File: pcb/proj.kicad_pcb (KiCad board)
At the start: 2 copper layers, 125 x 185 mm, 152 parts, among them J1 Conn_02x05_Odd_Even, Q1 MMBT3904, SW1 Reset, SW10 8, SW11 9, SW12 /, SW13 Deg/Rad, SW14 Clear, SW15 4, SW16 5, SW17 6, SW18 X, SW19 Constants, SW2 Y/Stats, SW20 Del, SW21 1, SW22 2, SW23 3, SW24 -, SW25 Alpha, SW26 (/), SW27 Sin(x)/Sin-1(x), SW28 Cos(x)/Cos-1(x), SW29 Tan(x)/Tan-1(x), SW3 ./,, SW30 +, SW31 2nd, SW32 Γ(x), SW33 x^y/y√x, SW34 x^2/√x, SW35 log(x)/ln(x), SW36 e^x/10^x, SW37 Graph, SW38 Programs, SW39 Left, SW4 0, SW40 Up, SW41 Right, SW42 Down, SW43 Power, SW44 FPU BOOT0, SW45 Reset, SW5 +/-, SW6 Solve/=, SW7 Sci/Norm, SW8 X/Matrix, SW9 7, U1 PIC16C74, U2 STM32F401RCTx, U3 74HC238, U4 ISL9111EH50Z-T7A, U5 SN74LVC1G32DBVR, U6 TPS61021A, U7 SiP32510DT, U8 SN74LV1T34DBV, U9 SN74LV1T34DBV, Y1 20MHz

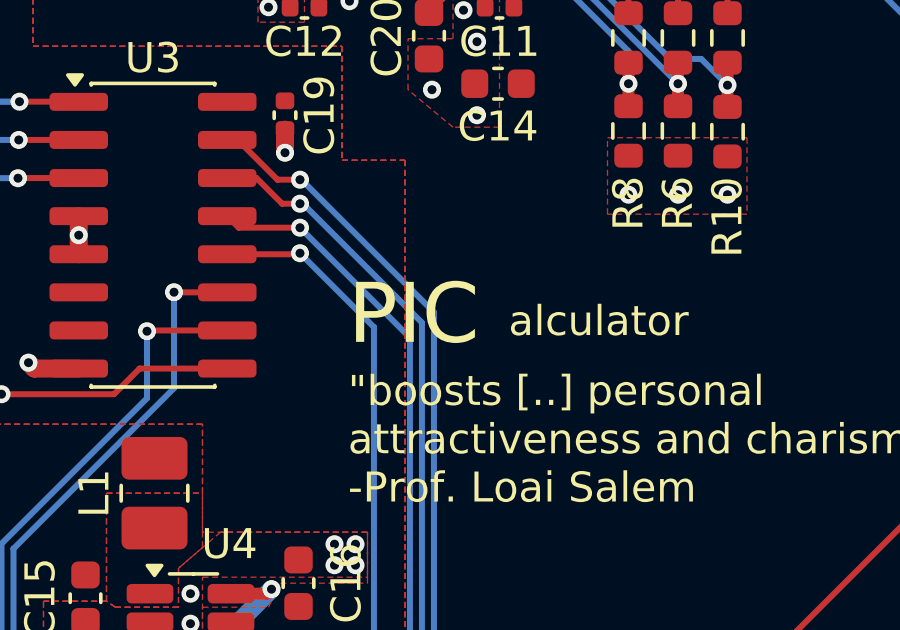
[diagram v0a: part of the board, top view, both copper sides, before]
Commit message: Update proj.kicad_pcb
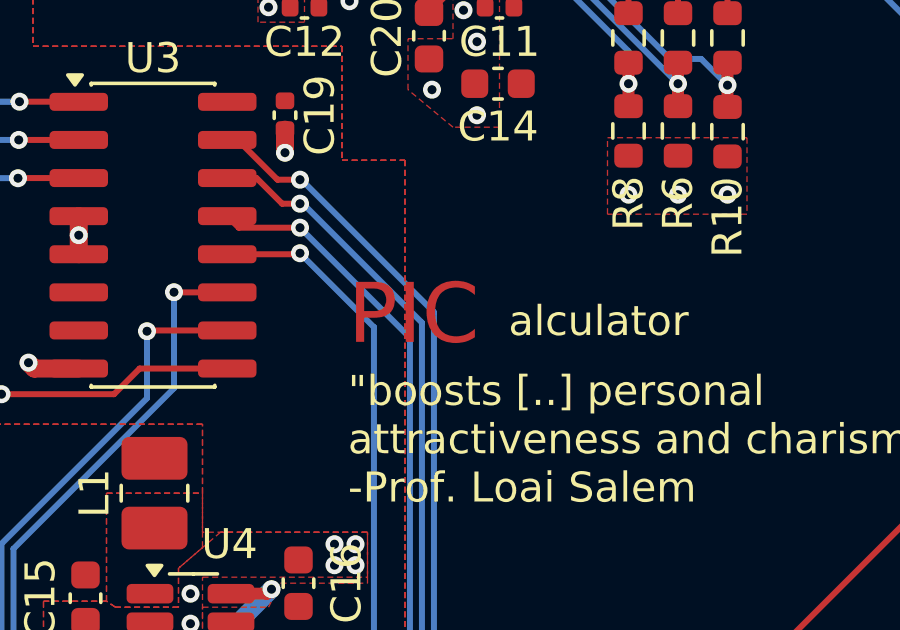
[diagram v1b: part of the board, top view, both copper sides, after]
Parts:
- D1, D10, D11, D12, D13, D14, D15, D16, D17, D18, D19, D2, D20, D21, D22, D23, D24, D25, D26, D27, D28, D29, D3, D30, D31, D32, D33, D34, D35, D36, D37, D38, D39, D4, D40, D41, D42, D5, D6, D7, D8, D9: value SMD1200PL-TP -> B5819W
